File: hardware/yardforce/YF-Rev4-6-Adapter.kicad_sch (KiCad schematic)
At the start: 34 parts, among them J1 USB_OTG, J2 JTAG ARM-10, J3 YF-Rev6-B, J4 YF-Rev6-A, J5 YF-Rev4-A, J6 YF-Rev4-B, J7 OM UI Board, U1 XC6220B331MR, U2 ESP32-S3-WROOM-1, U3 TCA9555PWR

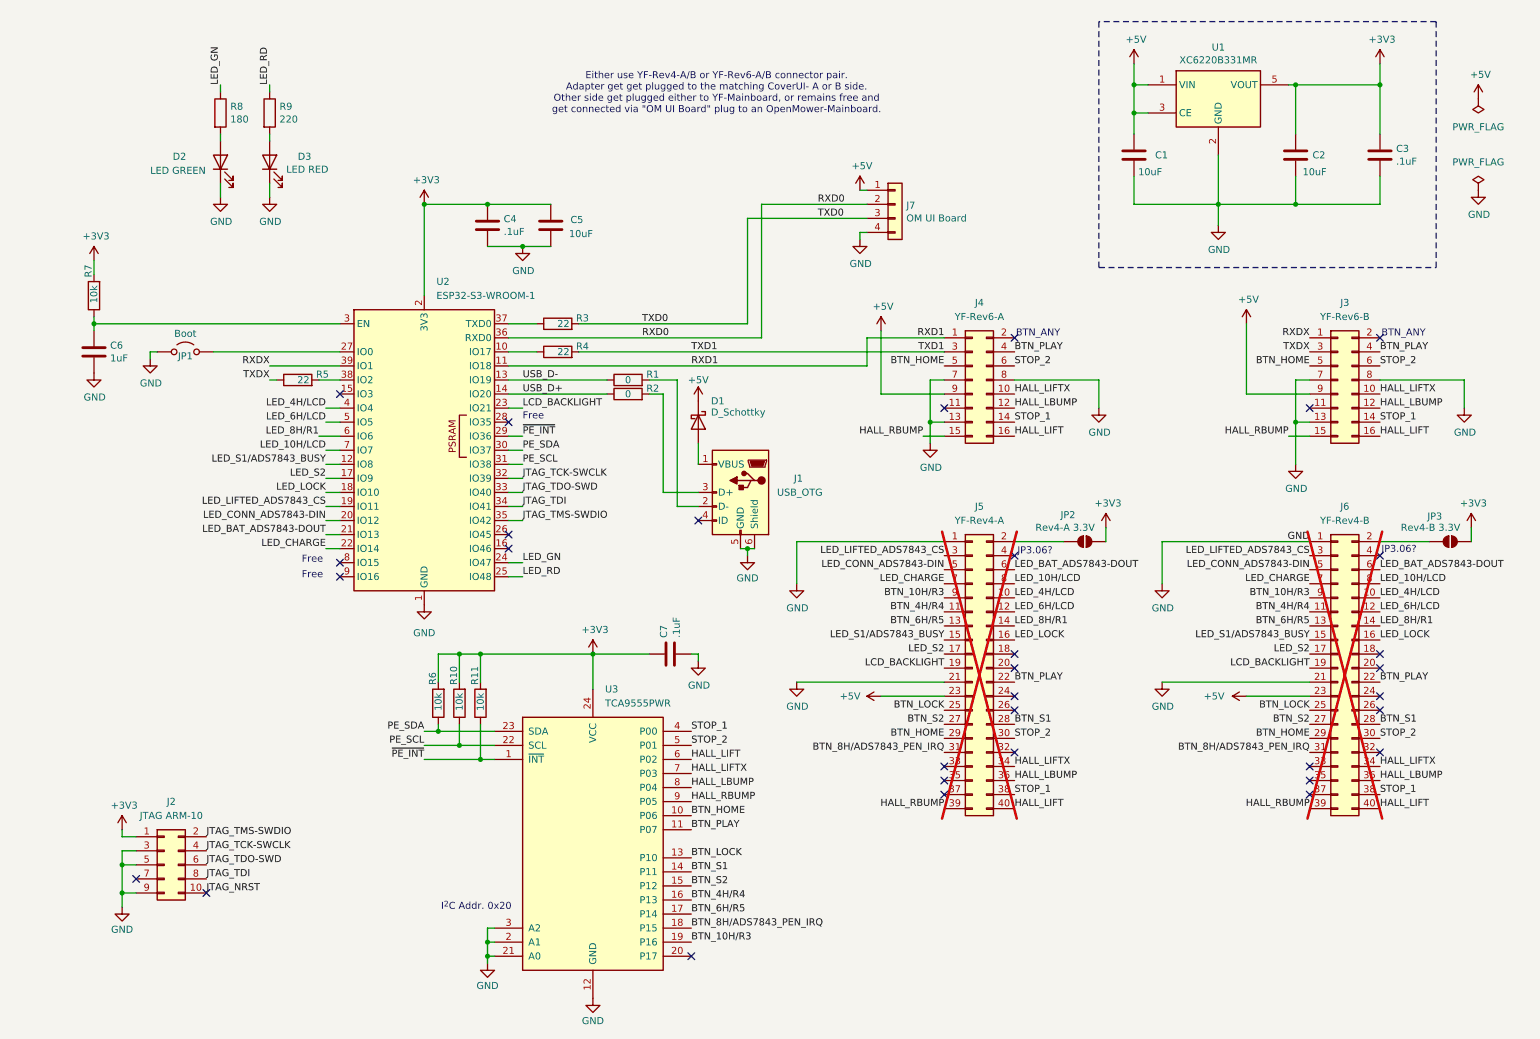
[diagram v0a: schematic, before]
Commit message: Add HW Prototype v0.1
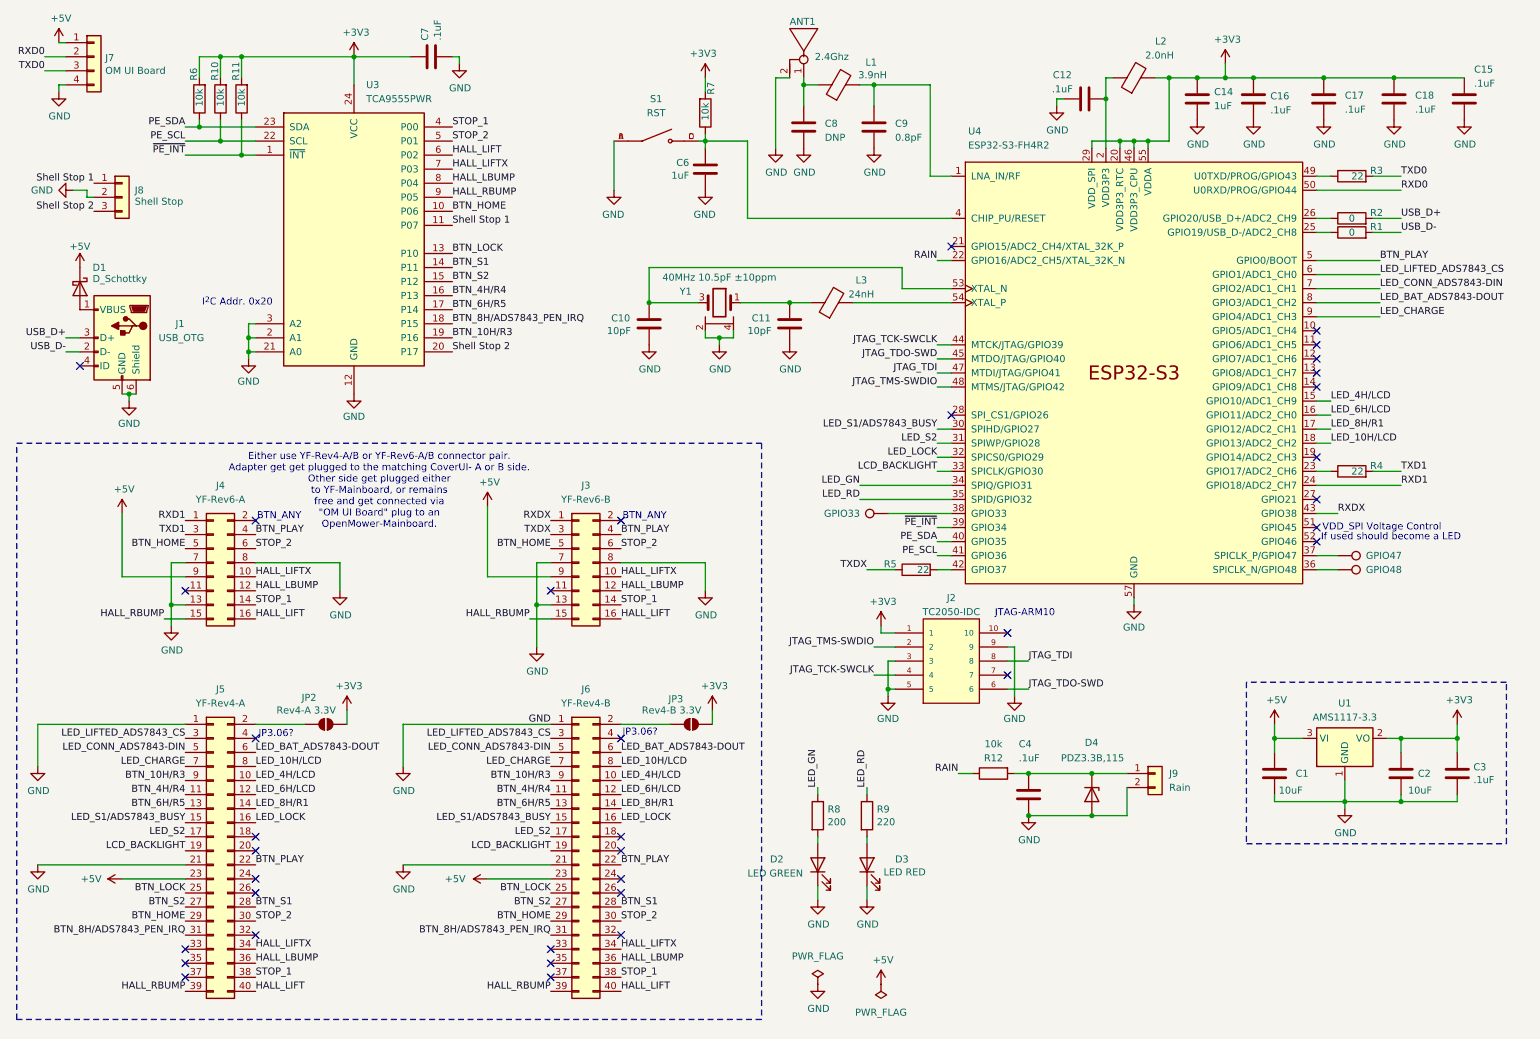
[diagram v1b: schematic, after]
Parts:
- removed C5: 10uF, Capacitor_SMD:C_0603_1608Metric, symbol Device:C
- removed J2: JTAG ARM-10, Connector_IDC:IDC-Header_2x05_P2.54mm_Vertical, symbol Connector_Generic:Conn_02x05_Odd_Even
- removed JP1: Boot, Connector_PinSocket_2.54mm:PinSocket_1x02_P2.54mm_Vertical, symbol Jumper:Jumper_2_Open
- removed U2: ESP32-S3-WROOM-1, libs:ESP32-S3-WROOM-1_MOD, symbol RF_Module:ESP32-S3-WROOM-1
- added ANT1: 2.4Ghz, libs:PCB_Antenna_2.4GHz_Left, symbol PCB_Antenna:PCB_Trace24
- added C10, C11: 10pF, Capacitor_SMD:C_0402_1005Metric, symbol Device:C
- added C12, C15, C16, C17, C18: .1uF, Capacitor_SMD:C_0402_1005Metric, symbol Device:C
- added C14: 1uF, Capacitor_SMD:C_0402_1005Metric, symbol Device:C
- added C8: DNP, Capacitor_SMD:C_0402_1005Metric, symbol Device:C
- added C9: 0.8pF, Capacitor_SMD:C_0402_1005Metric, symbol Device:C
- added D4: PDZ3.3B,115, Diode_SMD:D_SOD-323, symbol Device:D_Zener
- added GPIO33, GPIO47, GPIO48: TestPoint, TestPoint:TestPoint_Pad_1.0x1.0mm, symbol Connector:TestPoint
- added J2: TC2050-IDC, libs:TAG-CONNECT_TC2050-IDC, symbol TC2050-IDC:TC2050-IDC
- added J8: Shell Stop, Connector_JST:JST_XH_B3B-XH-A_1x03_P2.50mm_Vertical, symbol Connector_Generic:Conn_01x03
- added J9: Rain, Connector_JST:JST_XH_B2B-XH-A_1x02_P2.50mm_Vertical, symbol Connector_Generic:Conn_01x02
- added L1: 3.9nH, Inductor_SMD:L_0402_1005Metric, symbol Device:FerriteBead
- added L2: 2.0nH, Inductor_SMD:L_0402_1005Metric, symbol Device:FerriteBead
- added L3: 24nH, Inductor_SMD:L_0402_1005Metric, symbol Device:FerriteBead
- added R12: 10k, Resistor_SMD:R_0603_1608Metric, symbol Device:R
- added S1: RST, libs:SW_TS-1187A-B-A-B, symbol TS-1187A-B-A-B:TS-1187A-B-A-B
- added U4: ESP32-S3-FH4R2, Package_DFN_QFN:QFN-56-1EP_7x7mm_P0.4mm_EP4x4mm_ThermalVias, symbol PCM_Espressif:ESP32-S3
- added Y1: 40MHz 10.5pF ±10ppm, Crystal:Crystal_SMD_2016-4Pin_2.0x1.6mm, symbol Crystal_SMD:XRCGB40M000F4M02R0
- C1, C2: JLCPCB C76608 -> (none); LCSC (none) -> C19702
- C3, C7: JLCPCB C41851 -> (none); LCSC (none) -> C1525
- C4: JLC (none) -> C307331; JLCPCB C41851 -> (none); LCSC (none) -> C1525; Stock_PN C-402-.1uF-16V-X7R -> (none)
- C6: JLCPCB C76999 -> (none); LCSC (none) -> C52923
- D1: JLCPCB C82288 -> (none); LCSC (none) -> C82288
- D2: JLCPCB KT-0603G -> (none); LCSC (none) -> C12624
- D3: JLCPCB KT-0603R -> (none); LCSC (none) -> C2286
- J1: JLCPCB C668588 -> (none); LCSC (none) -> C668588
- J3: JLCPCB C3320355 / C601981 -> (none); LCSC (none) -> C3320355 / C601981
- J4: JLCPCB C3320355 -> (none); LCSC (none) -> C3320355
- J5: JLCPCB C5909928 / C3029524 -> (none); LCSC (none) -> C5909928 / C3029524; now fitted
- J6: JLCPCB C5909928 -> (none); LCSC (none) -> C5909928; now fitted
- R1, R2: footprint Resistor_SMD:R_0603_1608Metric -> Resistor_SMD:R_0402_1005Metric; JLCPCB C21189 -> (none); LCSC (none) -> C17168
- R10, R11, R6, R7: JLCPCB C15401 -> (none); LCSC (none) -> C25804
- R3, R4, R5: JLCPCB C23345 -> (none); LCSC (none) -> C23345
- R8: value 180 -> 200; LCSC (none) -> C8218; Part Number RC0603FR-07180RL -> (none); Stock_PN R-603-180-.1W-1% -> (none)
- R9: Digikey 311-220HRCT-ND -> (none); LCSC (none) -> C22962; Part Number RC0603FR-07220RL -> (none); Stock_PN R-603-220-.1W-1% -> (none)
- U1: value XC6220B331MR -> AMS1117-3.3; footprint Package_TO_SOT_SMD:SOT-23-5 -> Package_TO_SOT_SMD:SOT-223-3_TabPin2; symbol Regulator_Linear:XC6220B331MR -> Regulator_Linear:AMS1117-3.3; Digikey 893-1133-1-ND -> (none); LCSC C86534 -> C6186; Part Number XC6220B331MR -> (none); Stock_PN U-XC6220B331MR -> (none)
- U3: LCSC (none) -> C465732
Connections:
- net +3V3: now also U1.2 (VO), C14.1, C15.1, C16.1, C17.1, C18.1, J2.1, L2.2, U4.20 (VDD3P3_RTC), U4.29 (VDD_SPI), U4.46 (VDD3P3_CPU), U4.55 (VDDA), U4.56 (VDDA); no longer C4.1, U1.5 (VOUT)
- net +5V: no longer U1.1 (VIN)
- net BTN_PLAY: now also U4.5 (GPIO0/BOOT); no longer U3.11 (P07)
- net GND: now also U1.1 (GND), ANT1.2, C10.2, C11.2, C12.1, C14.2, C15.2, C16.2, C17.2, C18.2, C8.2, C9.2, D4.2 (A), J2.3, J2.5, J2.9, J8.2 (Pin_2), J9.2 (Pin_2), S1.A, S1.B, U4.57 (GND), Y1.2, Y1.4; no longer U1.2 (GND)
- net JTAG_TCK-SWCLK: now also J2.4, U4.44 (MTCK/JTAG/GPIO39)
- net JTAG_TDI: now also J2.8, U4.47 (MTDI/JTAG/GPIO41)
- net JTAG_TDO-SWD: now also J2.6, U4.45 (MTDO/JTAG/GPIO40)
- net JTAG_TMS-SWDIO: now also J2.2, U4.48 (MTMS/JTAG/GPIO42)
- net LCD_BACKLIGHT: now also U4.33 (SPICLK/GPIO30)
- net LED_10H/LCD: now also U4.18 (GPIO13/ADC2_CH2)
- net LED_4H/LCD: now also U4.15 (GPIO10/ADC1_CH9)
- net LED_6H/LCD: now also U4.16 (GPIO11/ADC2_CH0)
- net LED_8H/R1: now also U4.17 (GPIO12/ADC2_CH1)
- net LED_BAT_ADS7843-DOUT: now also U4.8 (GPIO3/ADC1_CH2)
- net LED_CHARGE: now also U4.9 (GPIO4/ADC1_CH3)
- net LED_CONN_ADS7843-DIN: now also U4.7 (GPIO2/ADC1_CH1)
- net LED_GN: now also U4.34 (SPIQ/GPIO31)
- net LED_LIFTED_ADS7843_CS: now also U4.6 (GPIO1/ADC1_CH0)
- net LED_LOCK: now also U4.32 (SPICS0/GPIO29)
- net LED_RD: now also U4.35 (SPID/GPIO32)
- net LED_S1/ADS7843_BUSY: now also U4.30 (SPIHD/GPIO27)
- net LED_S2: now also U4.31 (SPIWP/GPIO28)
- net PE_SCL: now also U4.41 (GPIO36)
- net PE_SDA: now also U4.40 (GPIO35)
- net RXD0: now also U4.50 (U0RXD/PROG/GPIO44)
- net RXD1: now also U4.24 (GPIO18/ADC2_CH7)
- net RXDX: now also U4.43 (GPIO38)
- net USB_D+: now also J1.3 (D+), R2.2; no longer R2.1
- net USB_D-: now also J1.2 (D-), R1.2; no longer R1.1
- net ~{PE_INT}: now also U4.39 (GPIO34)
- net at R5.2: now also U4.42 (GPIO37)
- net at C6.1, R7.1: now also S1.C, S1.D, U4.4 (CHIP_PU/RESET)
- net at R4.1: now also U4.23 (GPIO17/ADC2_CH6)
- net Shell Stop 2: now reaches U3.20 (P17)
- net Shell Stop 2: now also J8.3 (Pin_3)
- net at R3.1: now also U4.49 (U0TXD/PROG/GPIO43)
- new net: R2.1, U4.26 (GPIO20/USB_D+/ADC2_CH9)
- new net: C11.1, L3.1, Y1.1
- new net: C10.1, U4.53 (XTAL_N), Y1.3
- new net: C4.1, D4.1 (K), J9.1 (Pin_1), R12.2
- new net: ANT1.1, C8.1, L1.1
- new net: C9.1, L1.2, U4.1 (LNA_IN/RF)
- new net: R1.1, U4.25 (GPIO19/USB_D-/ADC2_CH8)
- new net: GPIO48.1, U4.36 (SPICLK_N/GPIO48)
- new net: GPIO47.1, U4.37 (SPICLK_P/GPIO47)
- new net: GPIO33.1, U4.38 (GPIO33)
- new net: L3.2, U4.54 (XTAL_P)
- new net RAIN: R12.1, U4.22 (GPIO16/ADC2_CH5/XTAL_32K_N)
- new net Shell Stop 1: J8.1 (Pin_1), U3.11 (P07)
- new net VDD3P3: C12.2, L2.1, U4.2 (VDD3P3), U4.3 (VDD3P3)
- no-connect marks 32 -> 36
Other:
- note added: "If used should become a LED"
- note added: "JTAG-ARM10"
- note added: "VDD_SPI Voltage Control"
- note removed: "Free"
- moved on the sheet: C1, C2, C3, C6, C7, D1, D2, D3, J1, J3, J4, J7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
